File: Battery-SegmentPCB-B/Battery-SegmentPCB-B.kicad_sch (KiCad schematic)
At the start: 10 parts, among them J11 Conn_01x04, J12 Conn_01x04, J13 Conn_01x04, J14 Conn_01x04, J15 Conn_01x04, J16 Conn_01x04, J17 Conn_01x04, J18 Conn_01x04, J19 Conn_01x09, J20 Conn_01x09

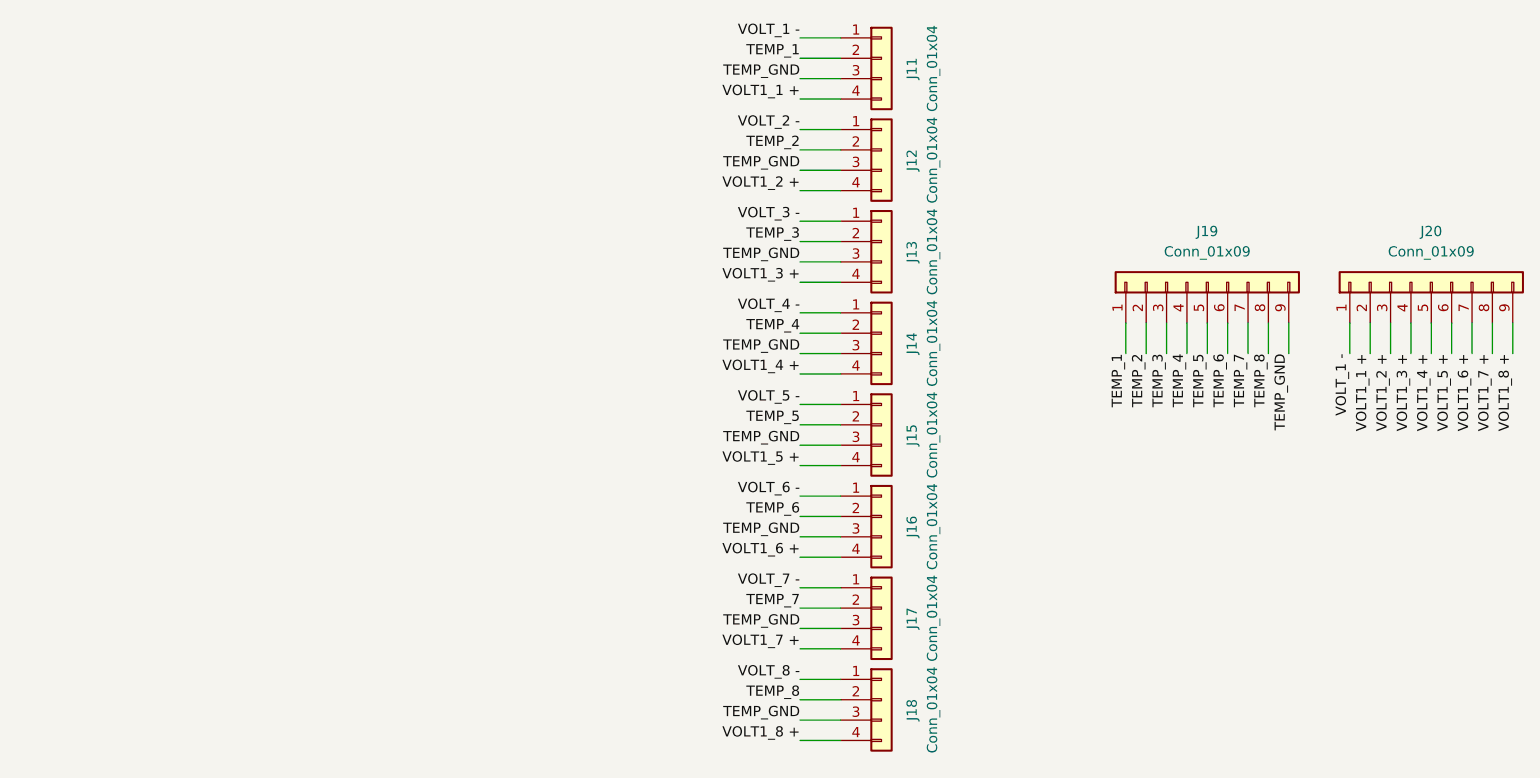
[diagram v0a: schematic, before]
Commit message: FUCK I FORGOT B
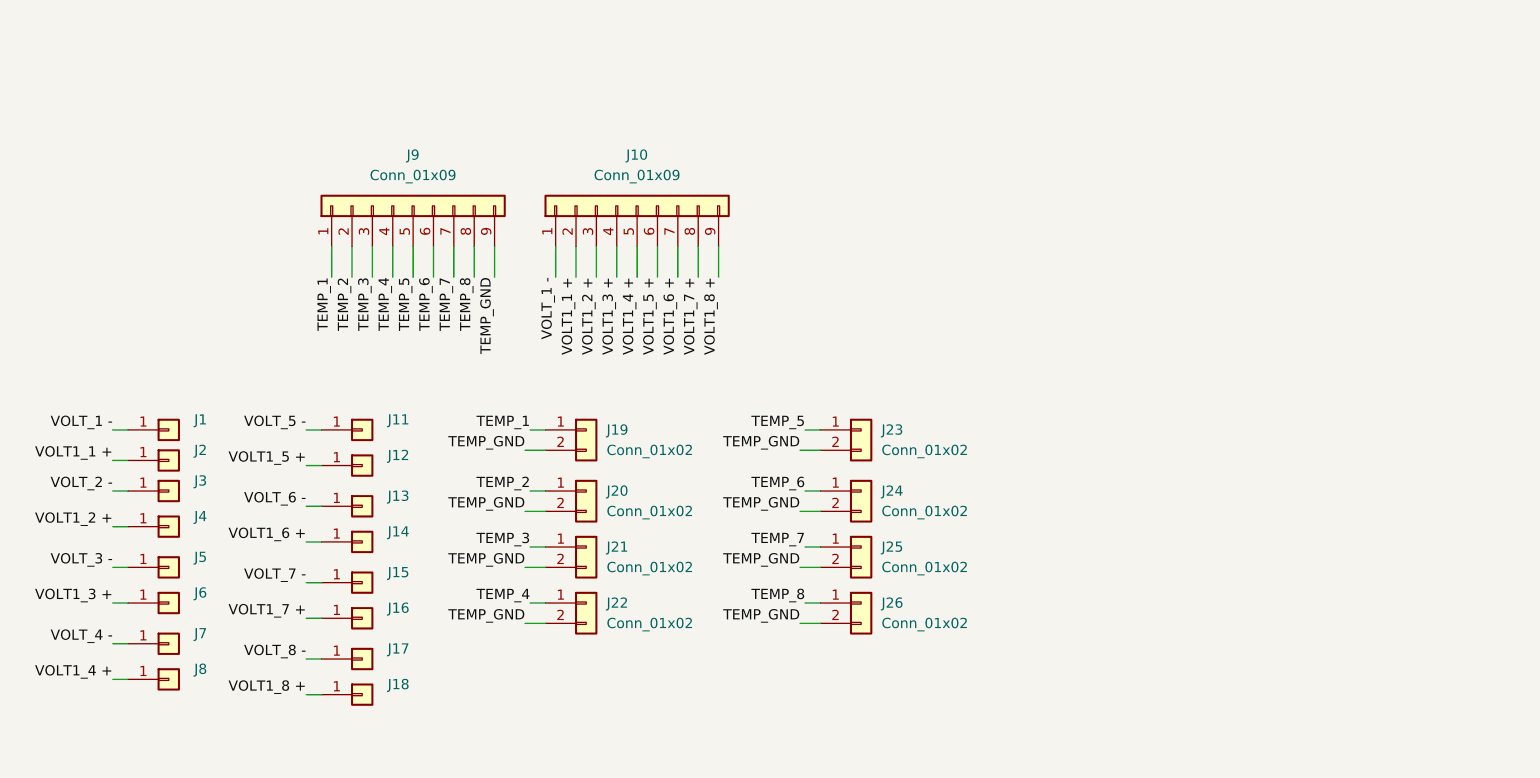
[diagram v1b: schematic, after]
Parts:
- removed J11, J12, J13, J14, J15, J16, J17, J18: Conn_01x04, footprints:CONN_S4B-PH-K-S_JST, symbol Connector_Generic:Conn_01x04
- removed J19, J20: Conn_01x09, footprints:CON_436500915_MOL, symbol Connector_Generic:Conn_01x09
- added J1, J11, J12, J13, J14, J15, J16, J17, J18, J2, J3, J4, J5, J6, J7, J8: Conn_01x01, MountingHole:MountingHole_3.2mm_M3_DIN965_Pad_TopOnly, symbol Connector_Generic:Conn_01x01
- added J10, J9: Conn_01x09, footprints:CON_436500915_MOL, symbol Connector_Generic:Conn_01x09
- added J19, J20, J21, J22, J23, J24, J25, J26: Conn_01x02, Connector_Molex:Molex_Nano-Fit_105309-xx02_1x02_P2.50mm_Vertical, symbol Connector_Generic:Conn_01x02
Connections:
- net TEMP_1: now also J19.1 (Pin_1), J9.1 (Pin_1)
- net TEMP_2: now also J20.1 (Pin_1), J9.2 (Pin_2)
- net TEMP_3: now also J21.1 (Pin_1), J9.3 (Pin_3)
- net TEMP_4: now also J22.1 (Pin_1), J9.4 (Pin_4)
- net TEMP_5: now also J23.1 (Pin_1), J9.5 (Pin_5)
- net TEMP_6: now also J24.1 (Pin_1), J9.6 (Pin_6)
- net TEMP_7: now also J25.1 (Pin_1), J9.7 (Pin_7)
- net TEMP_8: now also J26.1 (Pin_1), J9.8 (Pin_8)
- net TEMP_GND: now also J19.2 (Pin_2), J20.2 (Pin_2), J21.2 (Pin_2), J22.2 (Pin_2), J23.2 (Pin_2), J24.2 (Pin_2), J25.2 (Pin_2), J26.2 (Pin_2), J9.9 (Pin_9)
- net VOLT1_1 +: now also J10.2 (Pin_2), J2.1 (Pin_1)
- net VOLT1_2 +: now also J10.3 (Pin_3), J4.1 (Pin_1)
- net VOLT1_3 +: now also J10.4 (Pin_4), J6.1 (Pin_1)
- net VOLT1_4 +: now also J10.5 (Pin_5), J8.1 (Pin_1)
- net VOLT1_5 +: now also J10.6 (Pin_6), J12.1 (Pin_1)
- net VOLT1_6 +: now also J10.7 (Pin_7), J14.1 (Pin_1)
- net VOLT1_7 +: now also J10.8 (Pin_8), J16.1 (Pin_1)
- net VOLT1_8 +: now also J10.9 (Pin_9), J18.1 (Pin_1)
- net VOLT_1 -: now also J1.1 (Pin_1), J10.1 (Pin_1)
- net VOLT_2 -: now also J3.1 (Pin_1)
- net VOLT_3 -: now also J5.1 (Pin_1)
- net VOLT_4 -: now also J7.1 (Pin_1)
- net VOLT_5 -: now also J11.1 (Pin_1)
- net VOLT_6 -: now also J13.1 (Pin_1)
- net VOLT_7 -: now also J15.1 (Pin_1)
- net VOLT_8 -: now also J17.1 (Pin_1)
